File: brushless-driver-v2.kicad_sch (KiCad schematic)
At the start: 25 parts, among them J1 Conn_01x07_Socket, J2 encoder_r, J5 encoder_l, J6 PRG, U3 ESP32-WROOM-32E

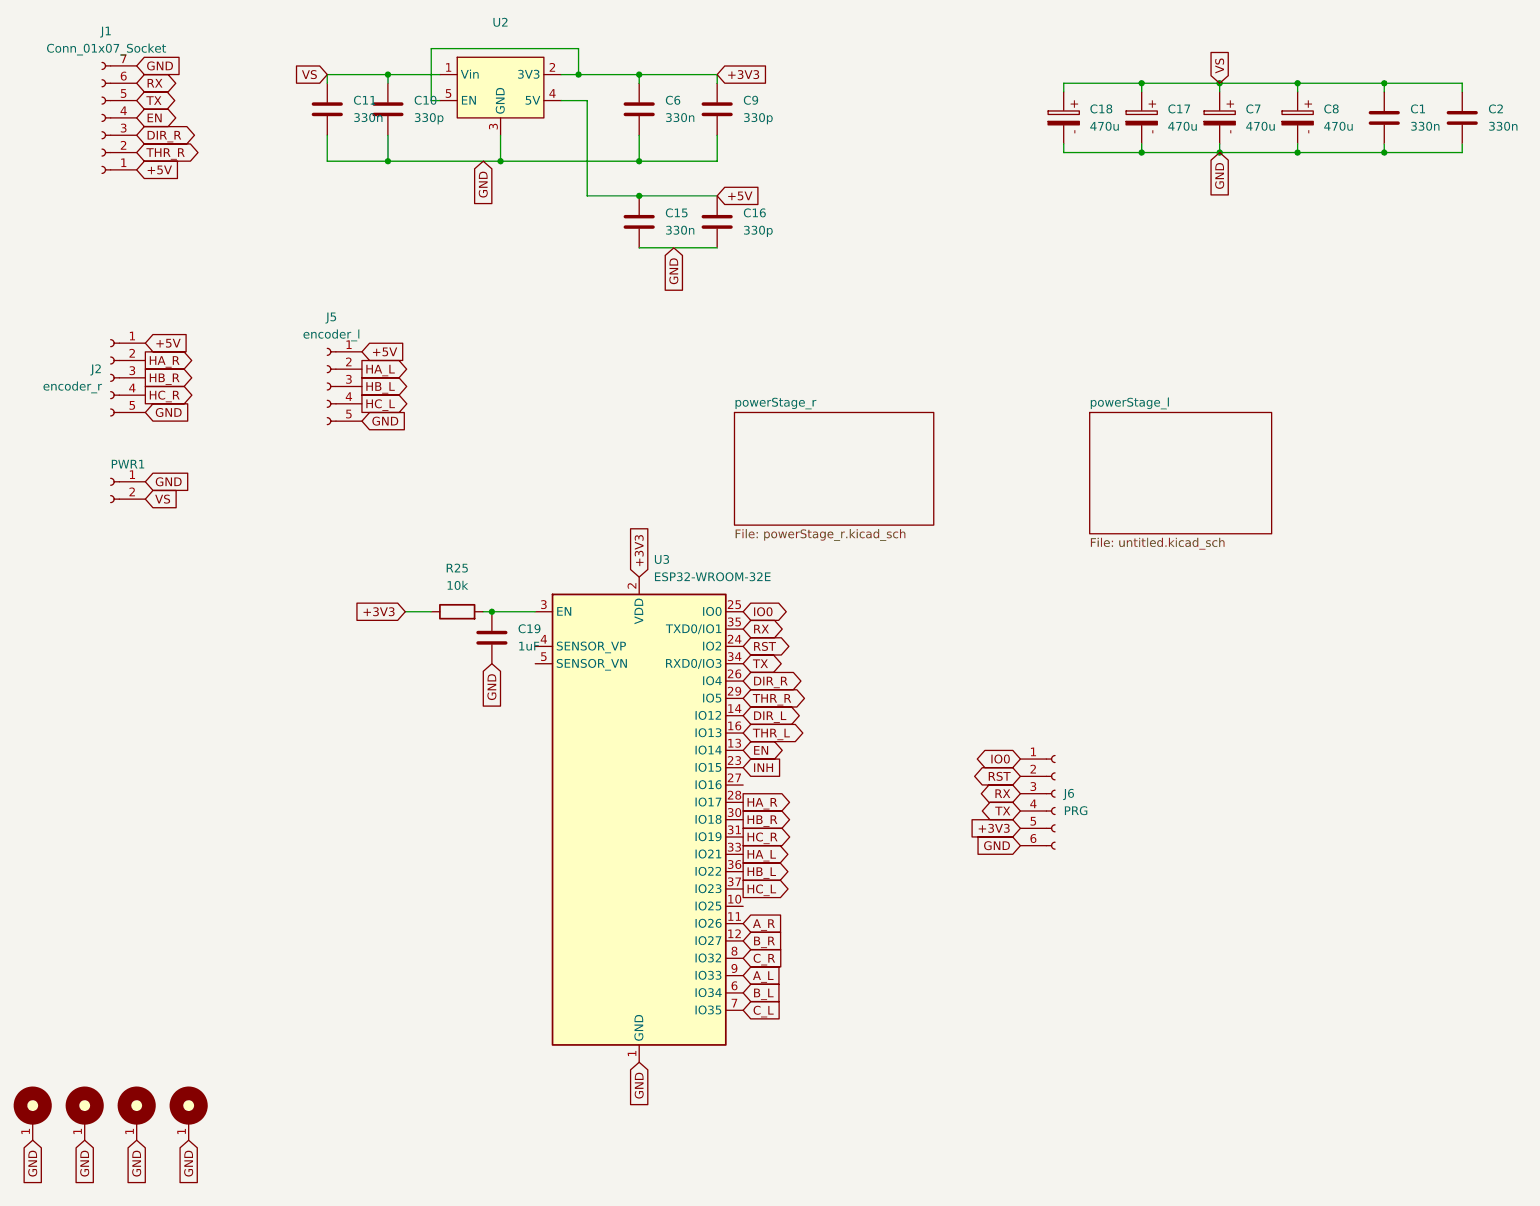
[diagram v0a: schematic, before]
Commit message: still unfinished
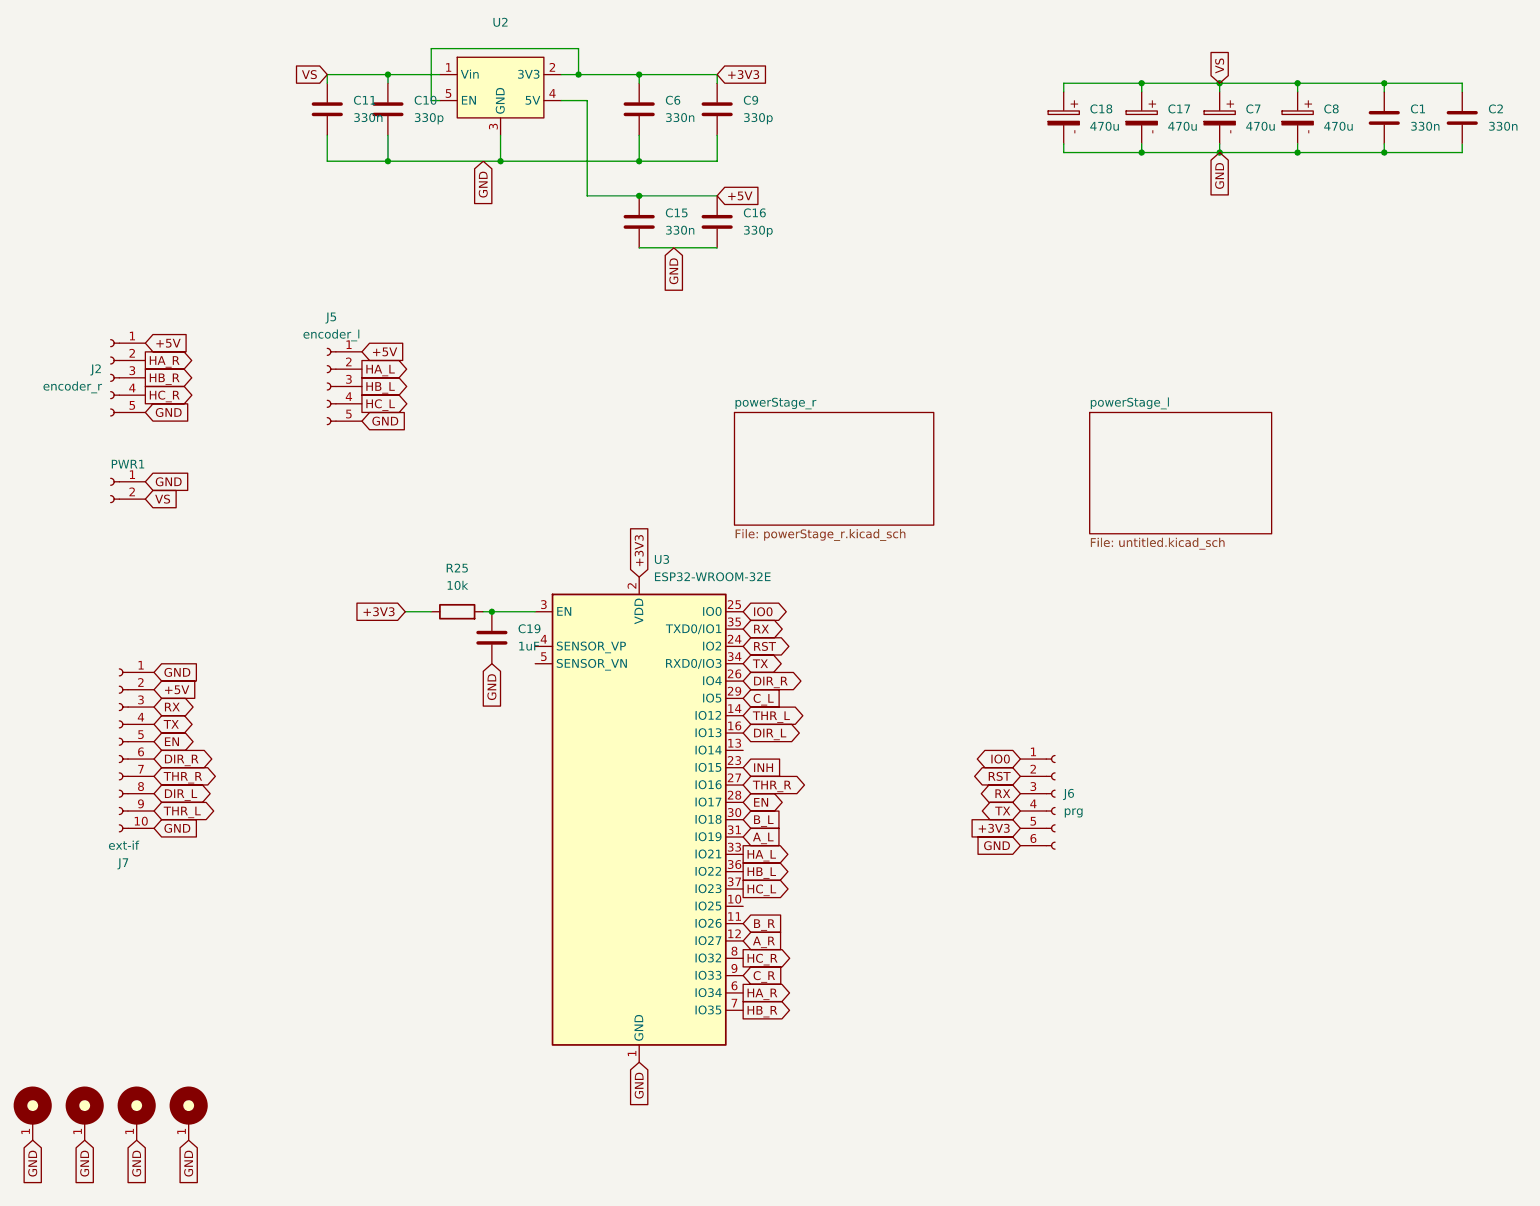
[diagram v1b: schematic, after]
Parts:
- removed J1: Conn_01x07_Socket, Connector_JST:JST_PH_S7B-PH-K_1x07_P2.00mm_Horizontal, symbol Connector:Conn_01x07_Socket
- added J7: ext-if, meiBib:Wannenstecker_10pin, symbol Connector:Conn_01x10_Socket
- J6: value PRG -> prg
- R25: footprint (none) -> Resistor_SMD:R_0805_2012Metric_Pad1.20x1.40mm_HandSolder
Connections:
- net +5V: now also J7.2 (Pin_2)
- net A_L: now also U3.31 (IO19); no longer U3.9 (IO33)
- net A_R: now also U3.12 (IO27); no longer U3.11 (IO26)
- net B_L: now also U3.30 (IO18); no longer U3.6 (IO34)
- net B_R: now also U3.11 (IO26); no longer U3.12 (IO27)
- net C_L: now also U3.29 (IO5); no longer U3.7 (IO35)
- net C_R: now also U3.9 (IO33); no longer U3.8 (IO32)
- net DIR_L: now also U3.16 (IO13), J7.8 (Pin_8); no longer U3.14 (IO12)
- net DIR_R: now also J7.6 (Pin_6)
- net EN: now also U3.28 (IO17), J7.5 (Pin_5); no longer U3.13 (IO14)
- net GND: now also J7.1 (Pin_1), J7.10 (Pin_10)
- net HA_R: now also U3.6 (IO34); no longer U3.28 (IO17)
- net HB_R: now also U3.7 (IO35); no longer U3.30 (IO18)
- net HC_R: now also U3.8 (IO32); no longer U3.31 (IO19)
- net RX: now also J7.3 (Pin_3)
- net THR_L: now also U3.14 (IO12), J7.9 (Pin_9); no longer U3.16 (IO13)
- net THR_R: now also U3.27 (IO16), J7.7 (Pin_7); no longer U3.29 (IO5)
- net TX: now also J7.4 (Pin_4)
